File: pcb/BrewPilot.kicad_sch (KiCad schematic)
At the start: 48 parts, among them J1 5V Power, J10 Boiler Probe, J11 SOL_L_FUSE, J12 5V_FUSE_5x20mm, J2 Flow Meter Group One, J3 Flow Meter Group Two, J4 FlexGPIO_1, J5 FlexGPIO_2, J6 RelayOut_1, J7 RelayOut2, J8 Solenoid Power, J9 Pump Power, K1 G3MB-202P DC5, K2 G3MB-202P DC5, K3 G3MB-202P DC5, K4 G3MB-202P DC5, K5 G3MB-202P DC5, Q1 BC547, Q2 BC547, Q3 BC547, Q4 BC547, Q5 BC547, U1 esp32

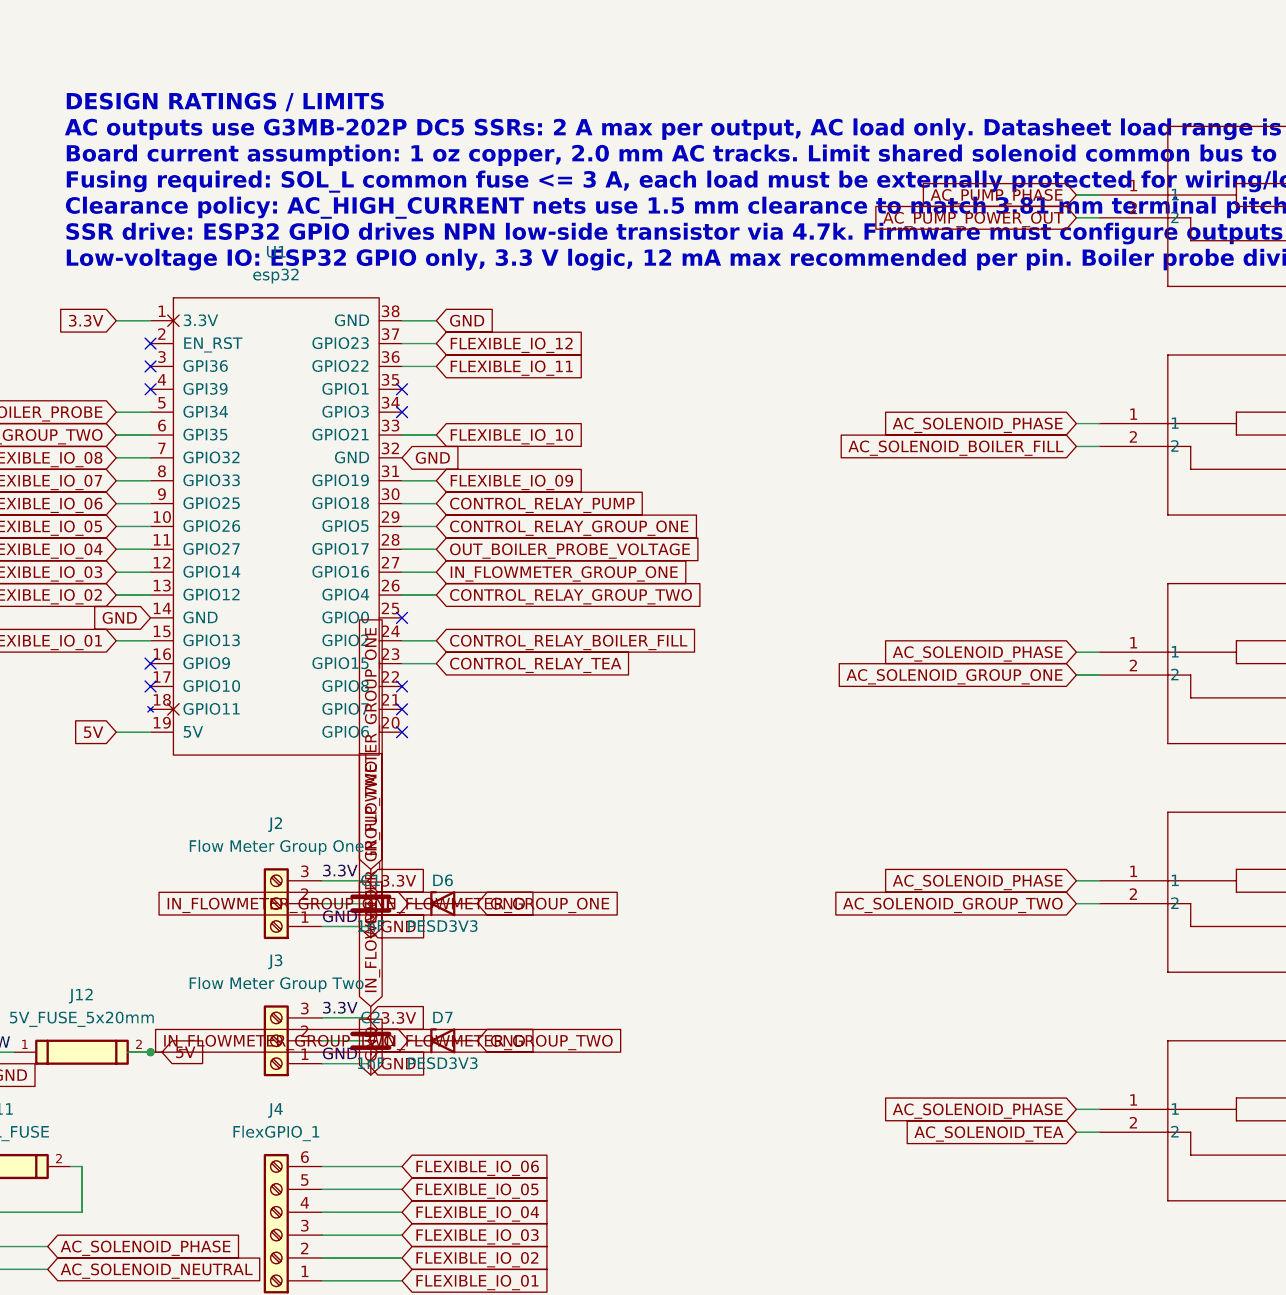
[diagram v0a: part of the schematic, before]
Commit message: stash
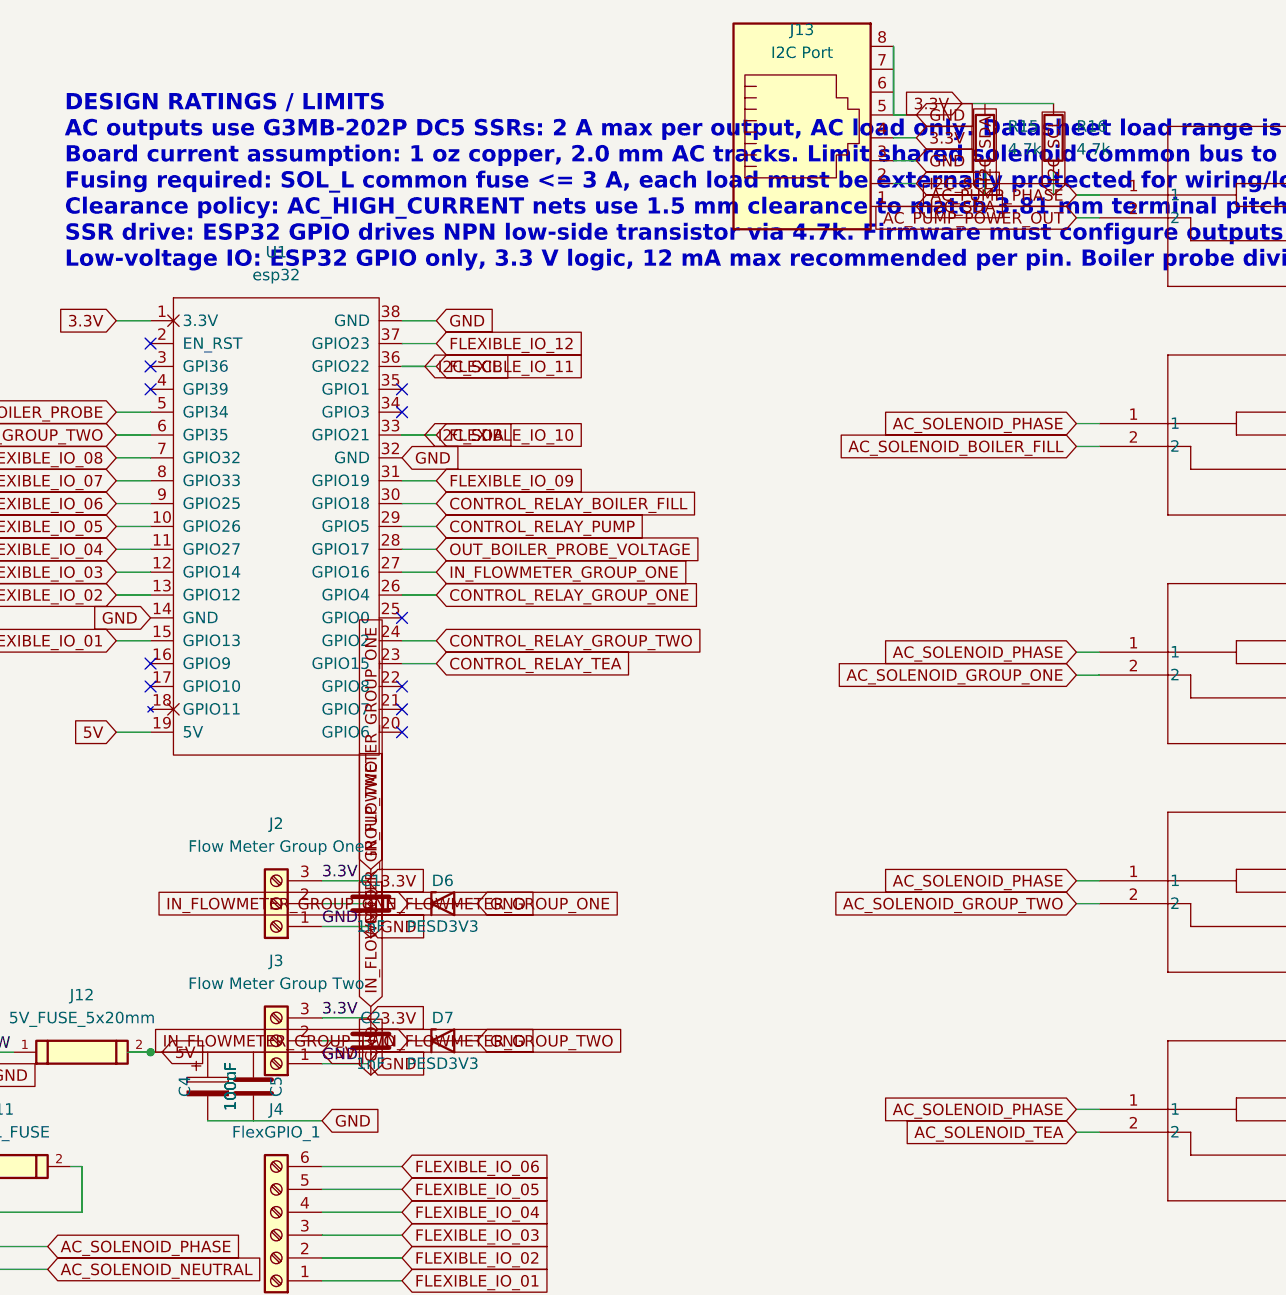
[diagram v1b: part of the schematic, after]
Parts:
- added C4: 100uF, Capacitor_THT:CP_Radial_D6.3mm_P2.50mm, symbol Device:C_Polarized
- added C5: 100nF, Capacitor_THT:C_Disc_D5.0mm_W2.5mm_P5.00mm, symbol Device:C
- added J13: I2C Port, Connector_RJ:RJ45_Amphenol_54602-x08_Horizontal, symbol Connector:8P8C
- added R15, R16: 4.7k, Resistor_THT:R_Axial_DIN0207_L6.3mm_D2.5mm_P7.62mm_Horizontal, symbol Device:R
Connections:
- net +3.3V: now also J13.4, R15.1, R16.1
- net +5V: now also C4.1, C5.1
- net CONTROL_RELAY_BOILER_FILL: now also U1.30 (GPIO18); no longer U1.24 (GPIO2)
- net CONTROL_RELAY_GROUP_ONE: now also U1.26 (GPIO4); no longer U1.29 (GPIO5)
- net CONTROL_RELAY_GROUP_TWO: now also U1.24 (GPIO2); no longer U1.26 (GPIO4)
- net CONTROL_RELAY_PUMP: now also U1.29 (GPIO5); no longer U1.30 (GPIO18)
- net FLEXIBLE_IO_10: now also J13.1, R15.2
- net FLEXIBLE_IO_11: now also J13.2, R16.2
- net GND: now also C4.2, C5.2, J13.3, J13.5, J13.6, J13.7, J13.8
